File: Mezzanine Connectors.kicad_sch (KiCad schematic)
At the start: 2 parts, among them J1000 10144518-082802LF, J1001 10144518-082802LF

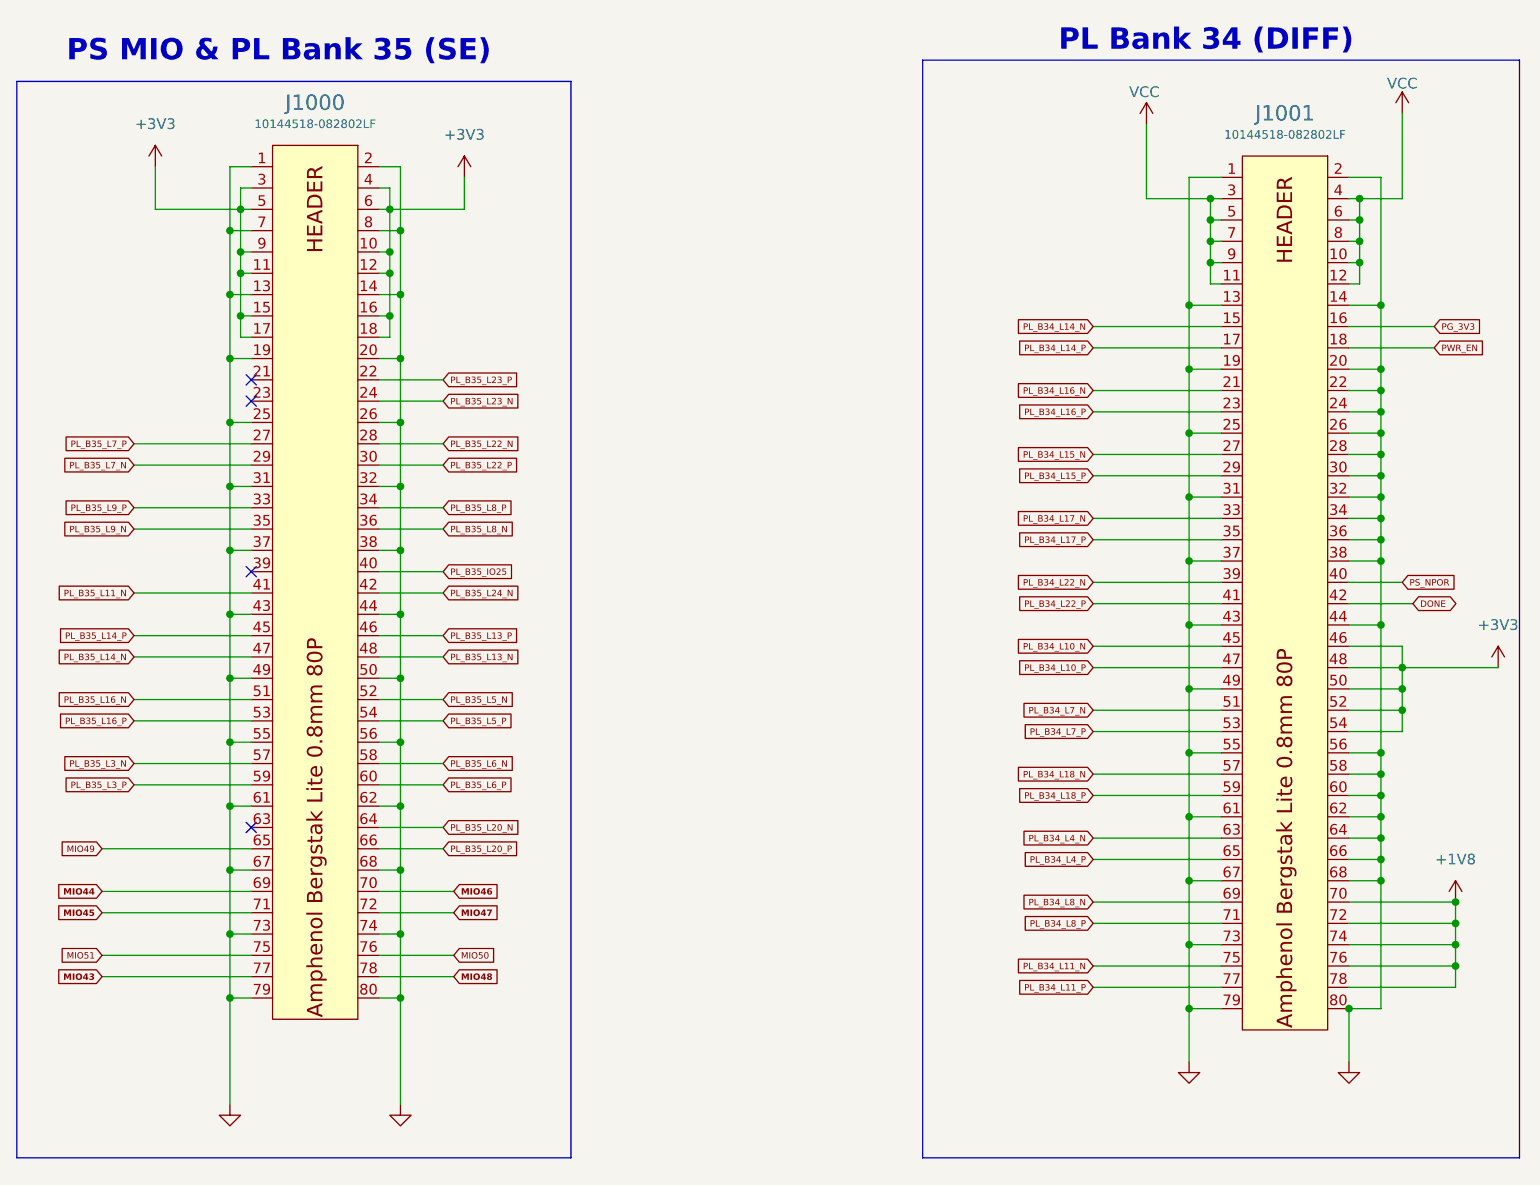
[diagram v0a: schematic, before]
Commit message: zynq_soc_complete_hdmi
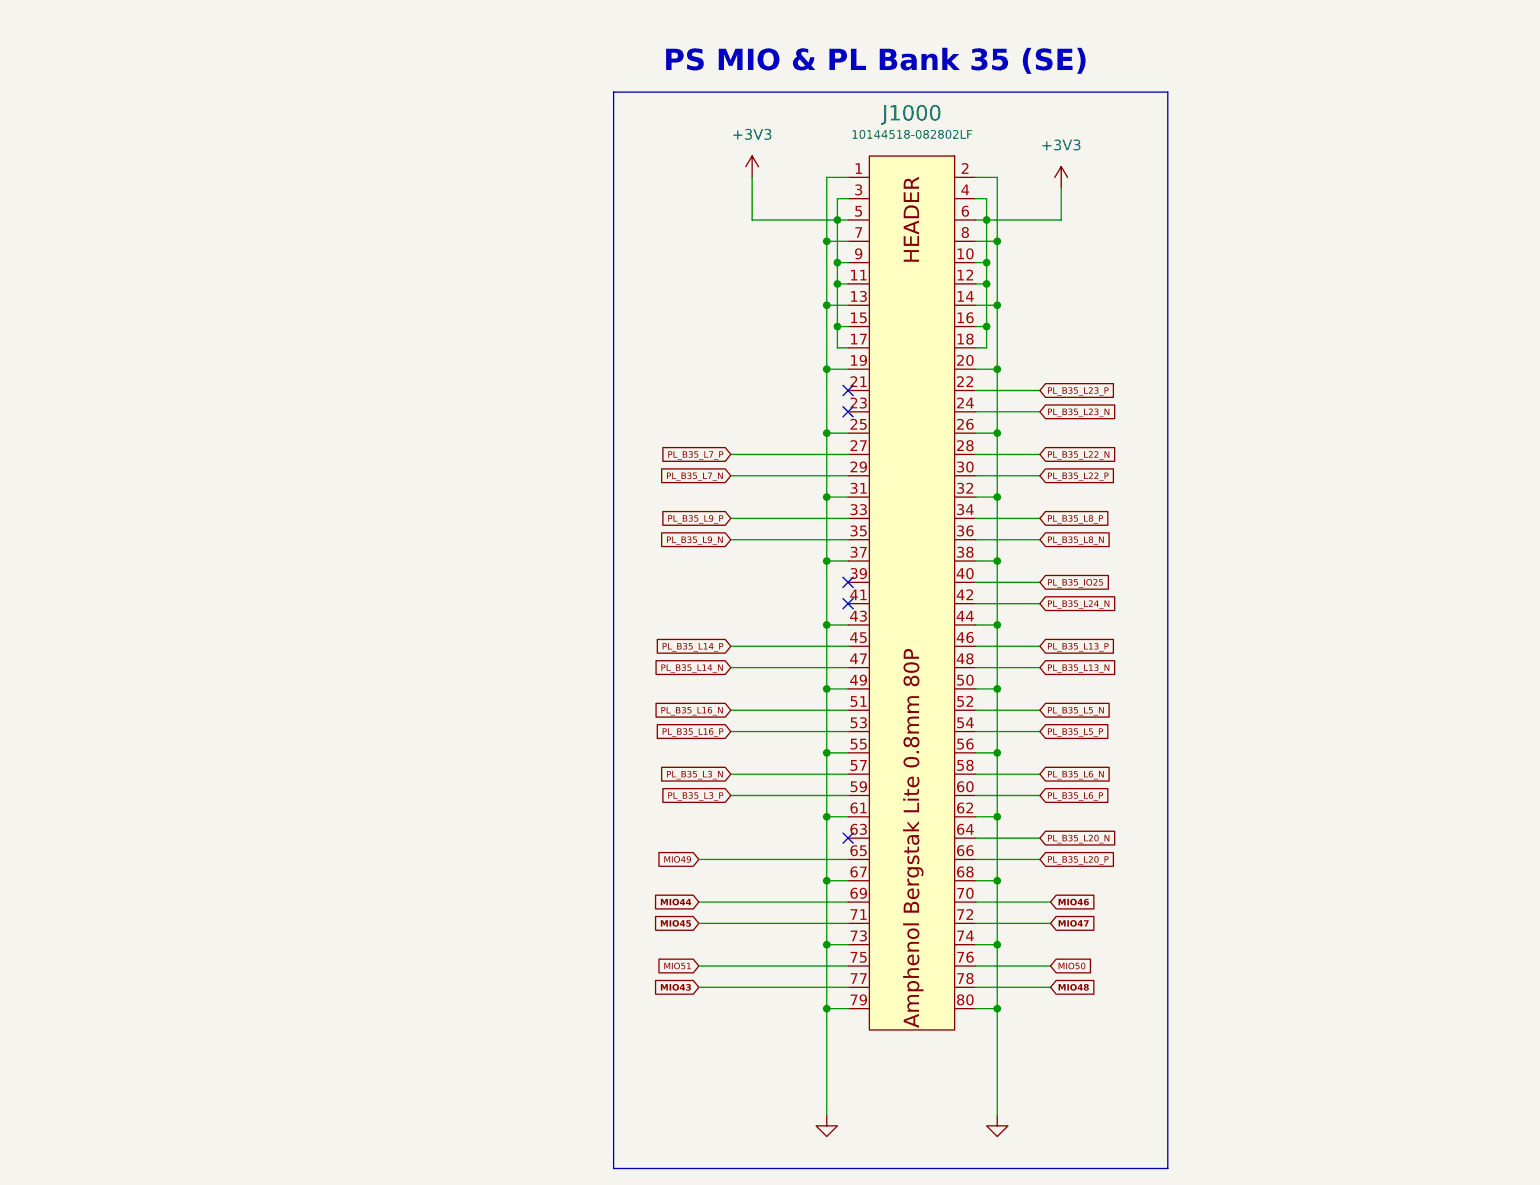
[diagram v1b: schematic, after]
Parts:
- removed J1001: 10144518-082802LF, Footprint-Lib-PhilsLab:10144518-082802LF, symbol Schematic-Lib-PhilsLab:10144518-082802LF
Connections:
- net PL_B35_L11_N: no longer names the net of J1000.41
- no-connect marks 4 -> 5
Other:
- note removed: "PL Bank 34 (DIFF)"
- moved on the sheet: J1000
